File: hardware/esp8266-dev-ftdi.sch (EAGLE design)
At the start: 61 parts, among them CON1 USBMICRO-NO_CENTER-LONG_PADS

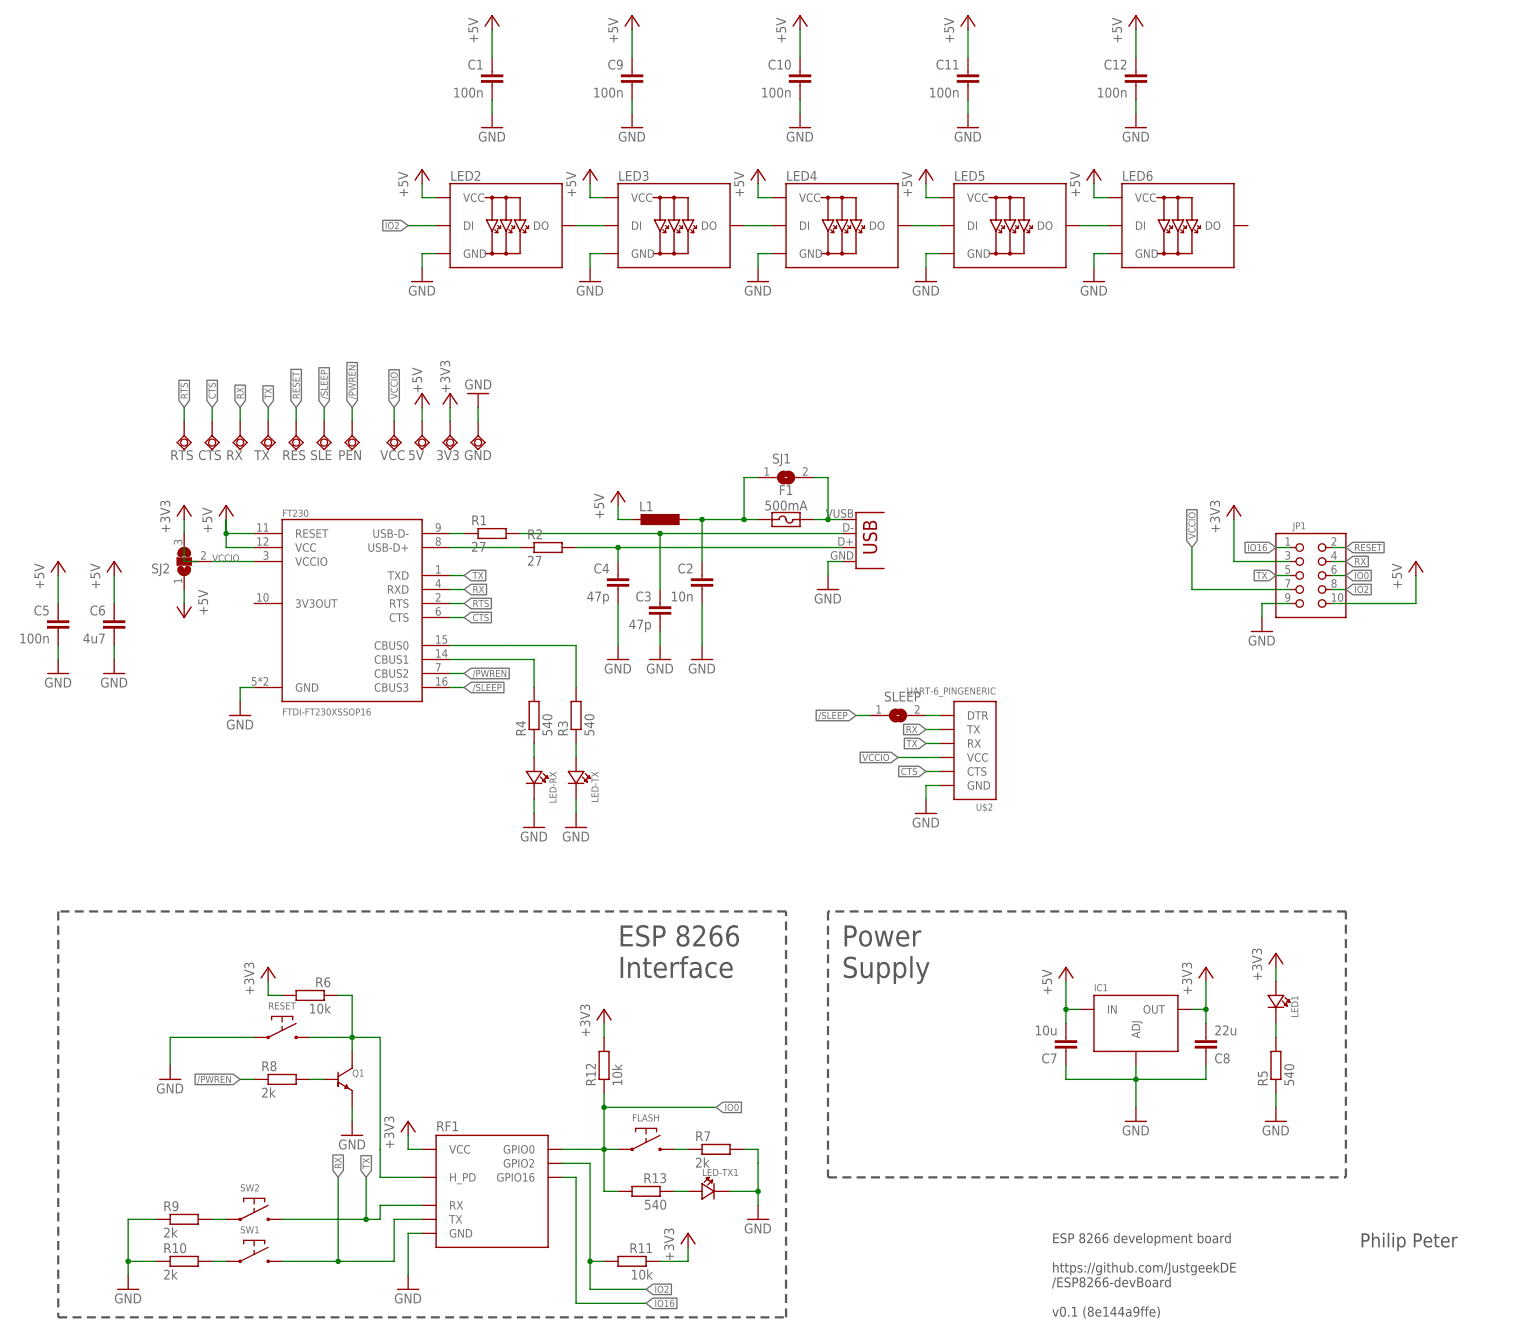
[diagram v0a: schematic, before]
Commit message: cleanup schematict
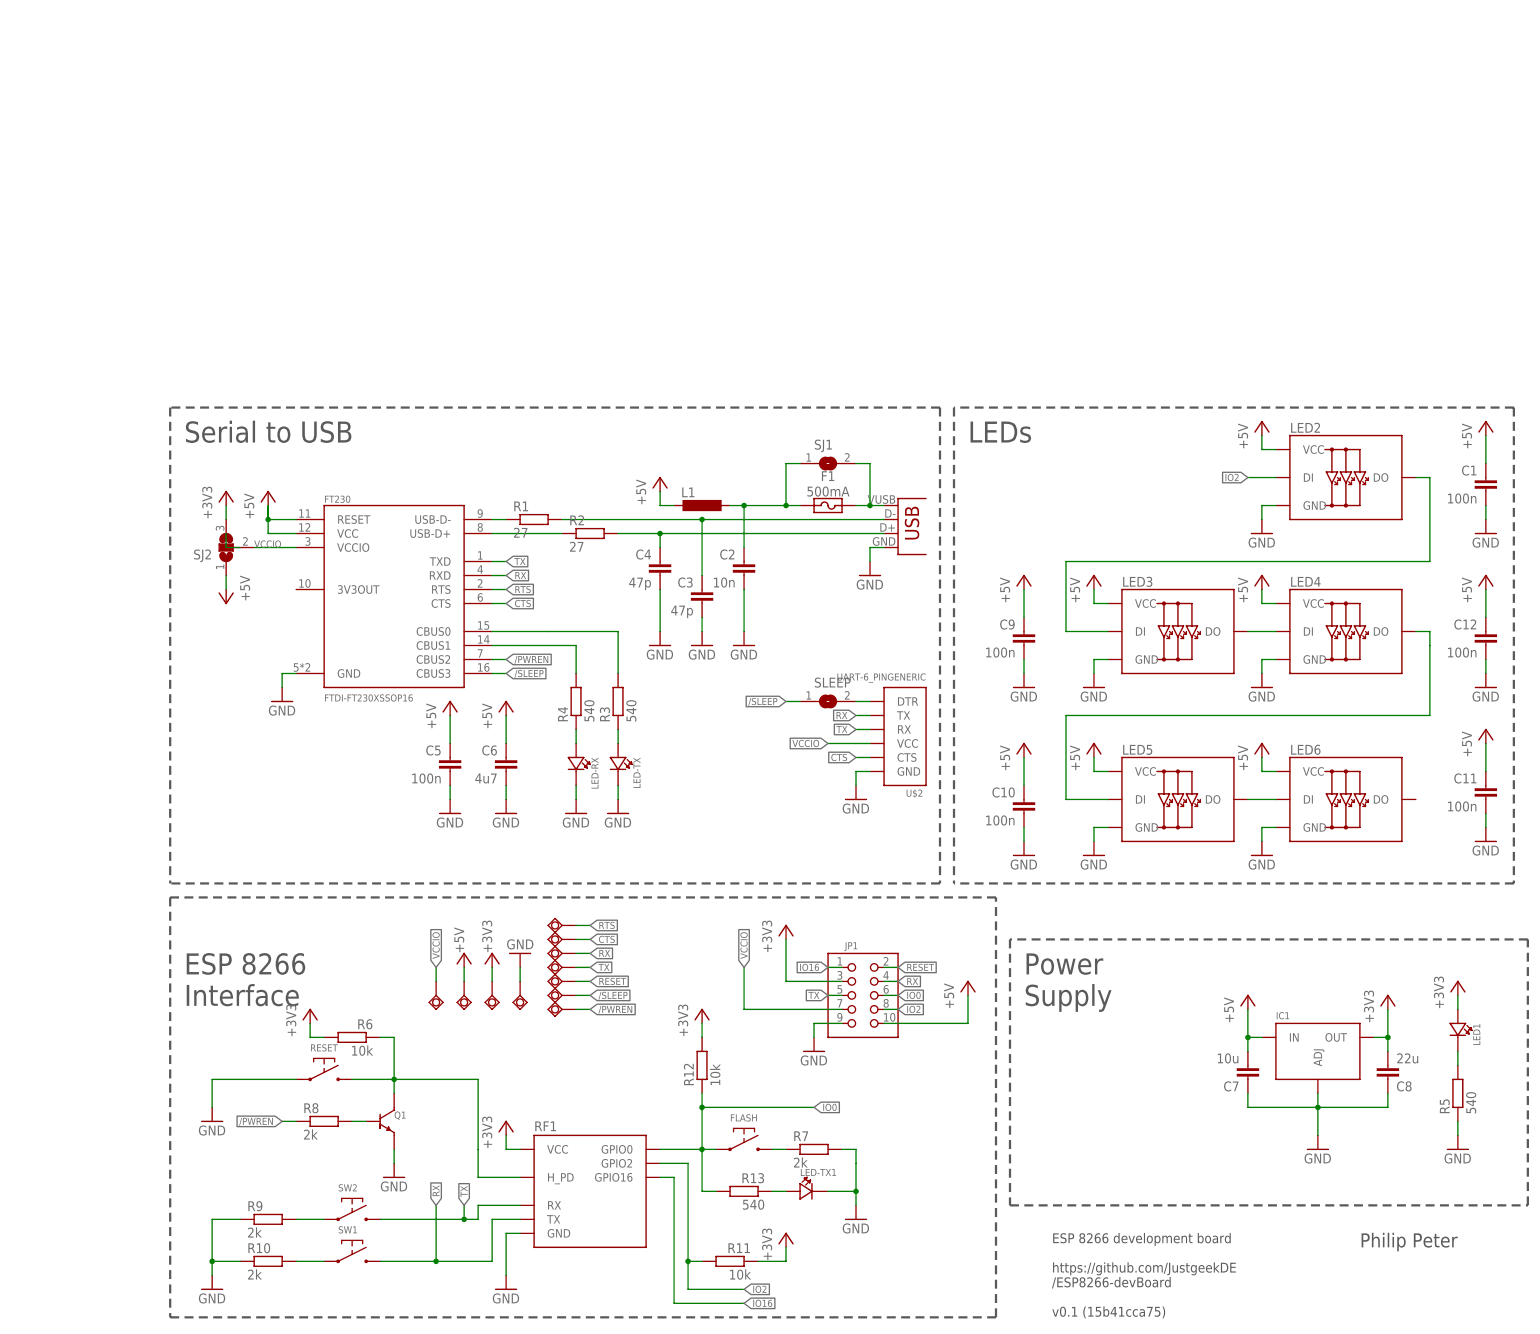
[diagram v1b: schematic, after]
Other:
- note added: "ESP 8266 development board https://github.com/JustgeekDE /ESP8266-devBoard v0.1 (15b41cca75)"
- note added: "LEDs"
- note added: "Serial to USB"
- note removed: "ESP 8266 development board https://github.com/JustgeekDE /ESP8266-devBoard v0.1 (8e144a9ffe)"
- moved on the sheet: C1, C10, C11, C12, C2, C3, C4, C5, C6, C7, C8, C9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
